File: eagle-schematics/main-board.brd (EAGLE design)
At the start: 49.5 x 50.8 mm, 26 parts

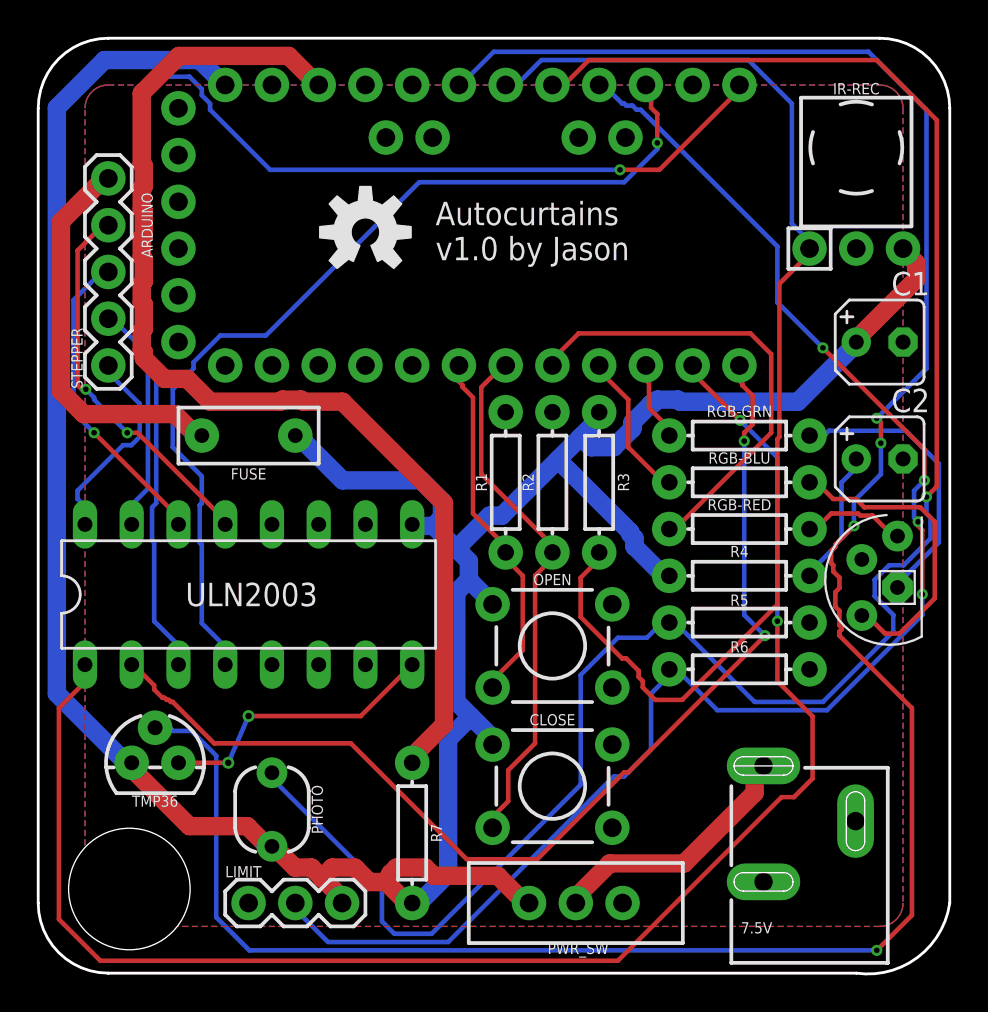
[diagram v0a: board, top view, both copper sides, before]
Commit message: Updated PCB design
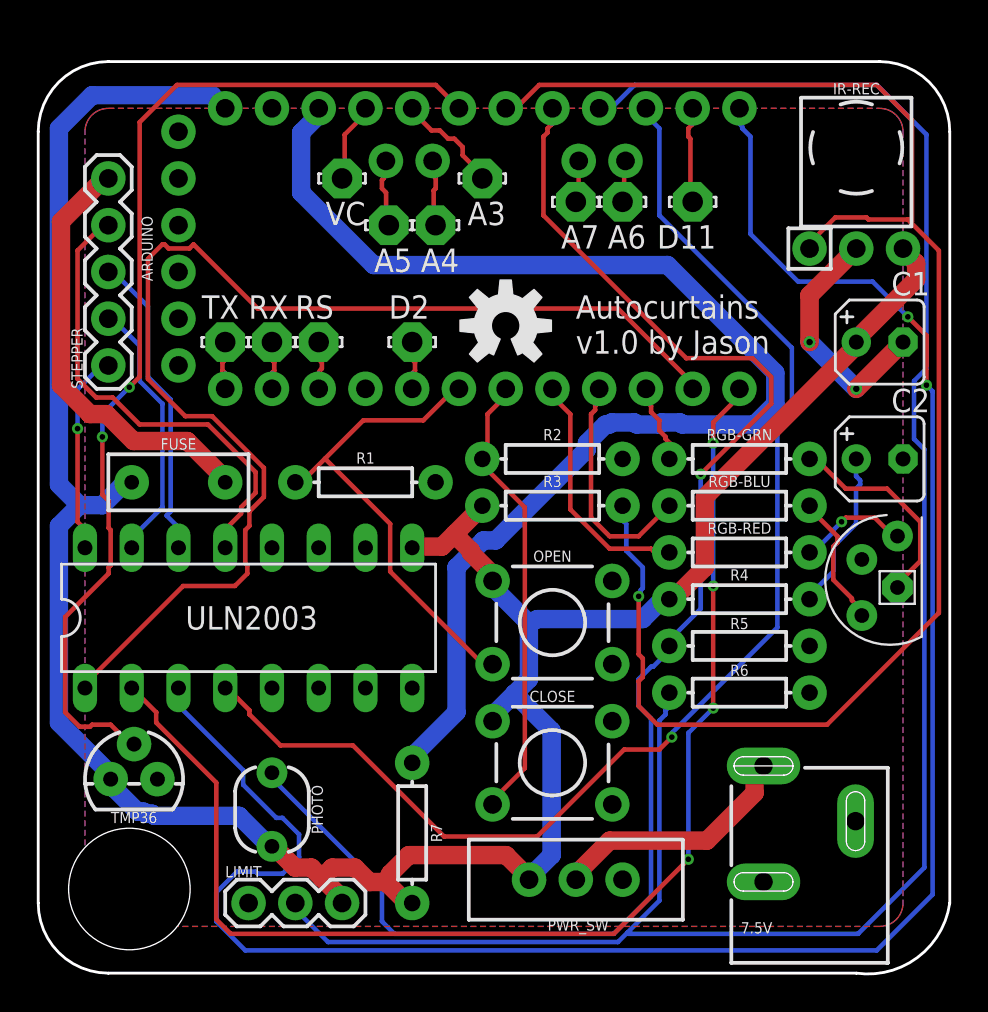
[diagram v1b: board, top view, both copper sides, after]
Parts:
- added A3, A4, A5, A6, A7, D11, D2, RS, RX, TX, VC: LSP11, solpad:LSP11
- moved U$1 9.16 mm to (25.4, 35.2)
- moved R1 7.62 mm to (17.8, 26.7), turned to 0 degrees
- moved FUSE 4.58 mm to (7.62, 26.7), turned to 0 degrees
- moved R3 2.84 mm to (27.9, 25.4), turned to 0 degrees
- moved TMP36 1.45 mm to (5.21, 10.5)
- moved ARDUINO 1.27 mm to (22.9, 39.4)
- moved RGB-BLU 1.27 mm to (38.1, 25.4)
- moved ULN2003 1.27 mm to (11.4, 19.3)
- moved R6 1.27 mm to (38.1, 15.2)
- moved PWR_SW 1.27 mm to (29.2, 5.08)
- moved CLOSE 1.27 mm to (27.9, 11.4)
- moved OPEN 1.27 mm to (27.9, 19.1)
- moved R2 1.27 mm to (27.9, 27.9), turned to 0 degrees
- moved R4 1.27 mm to (38.1, 20.3)
- moved R5 1.27 mm to (38.1, 17.8)
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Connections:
- removed net VCC: ARDUINO.21
- new net N$10: A6.MP, ARDUINO.A6
- new net N$11: A7.MP, ARDUINO.A7
- new net N$12: A5.MP, ARDUINO.A5
- new net N$13: A4.MP, ARDUINO.A4
- new net N$14: A3.MP, ARDUINO.20
- new net N$15: ARDUINO.21, VC.MP
- new net N$16: ARDUINO.5, D2.MP
- new net N$17: ARDUINO.3, RS.MP
- new net N$18: ARDUINO.2, RX.MP
- new net N$19: ARDUINO.1, TX.MP
- new net N$20: ARDUINO.14, D11.MP
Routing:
- net A2: track 127.7 -> 57.4 mm, vias 4 -> 2
- net D10: track 69.1 -> 109.3 mm, vias 1 -> 2
- net D13: track 83.7 -> 110.8 mm, vias 4 -> 0
- net A0: track 105.5 -> 79.9 mm
- net A1: track 64.5 -> 88.2 mm, vias 0 -> 1
- net D8: track 85.6 -> 66.1 mm, vias 2 -> 0
- net 5V: track 162.3 -> 143.7 mm
- net D12: track 51.9 -> 70.1 mm
- net D5: track 25.3 -> 13.3 mm
- net N$3: track 17.0 -> 7.40 mm
- net D9: track 59.6 -> 68.9 mm, vias 2 -> 4
- net AFTER: track 60.4 -> 69.5 mm
- net D3: track 19.7 -> 26.3 mm
- net N$14: track 0.00 -> 5.86 mm
- net N$20: track 0.00 -> 5.27 mm
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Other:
- board size 49.5 x 50.8 mm -> 49.5 x 49.6 mm
